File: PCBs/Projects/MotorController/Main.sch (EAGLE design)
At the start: 24 parts, among them Q1 ZXMP10A17GQ, Q2 BUK9240-100A.118, Q3 BUK9240-100A.118, Q4 MMBT5551LT1G, U1 LT4356-2

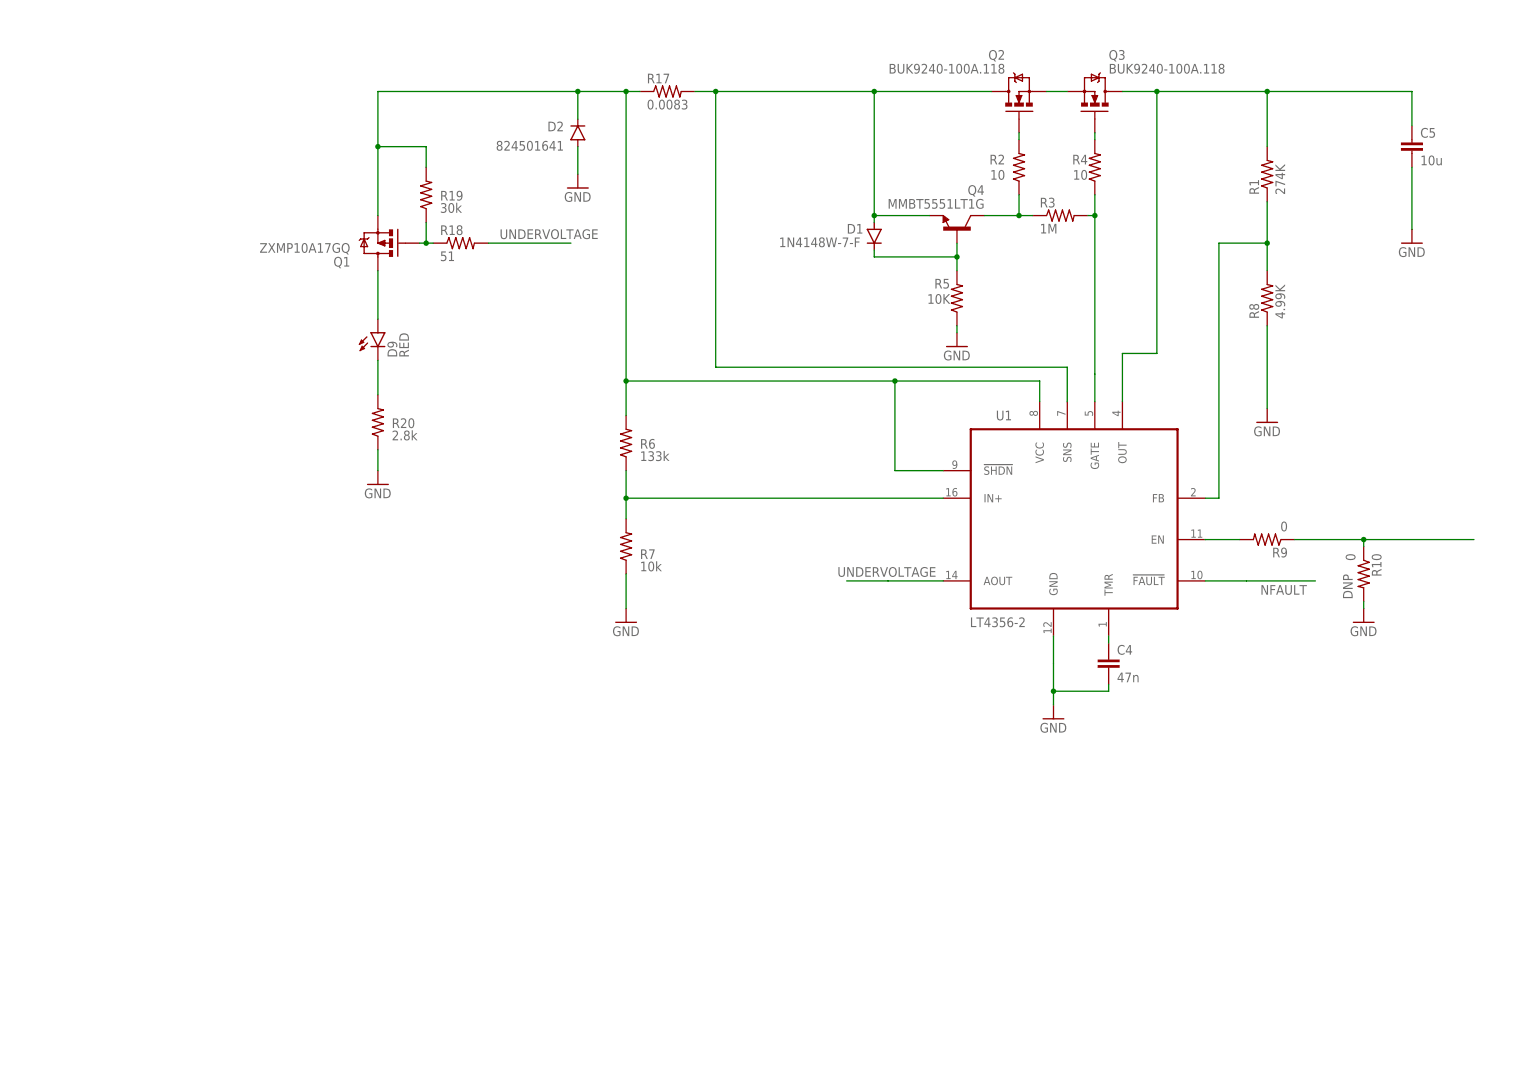
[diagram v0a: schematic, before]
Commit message: RepoFix
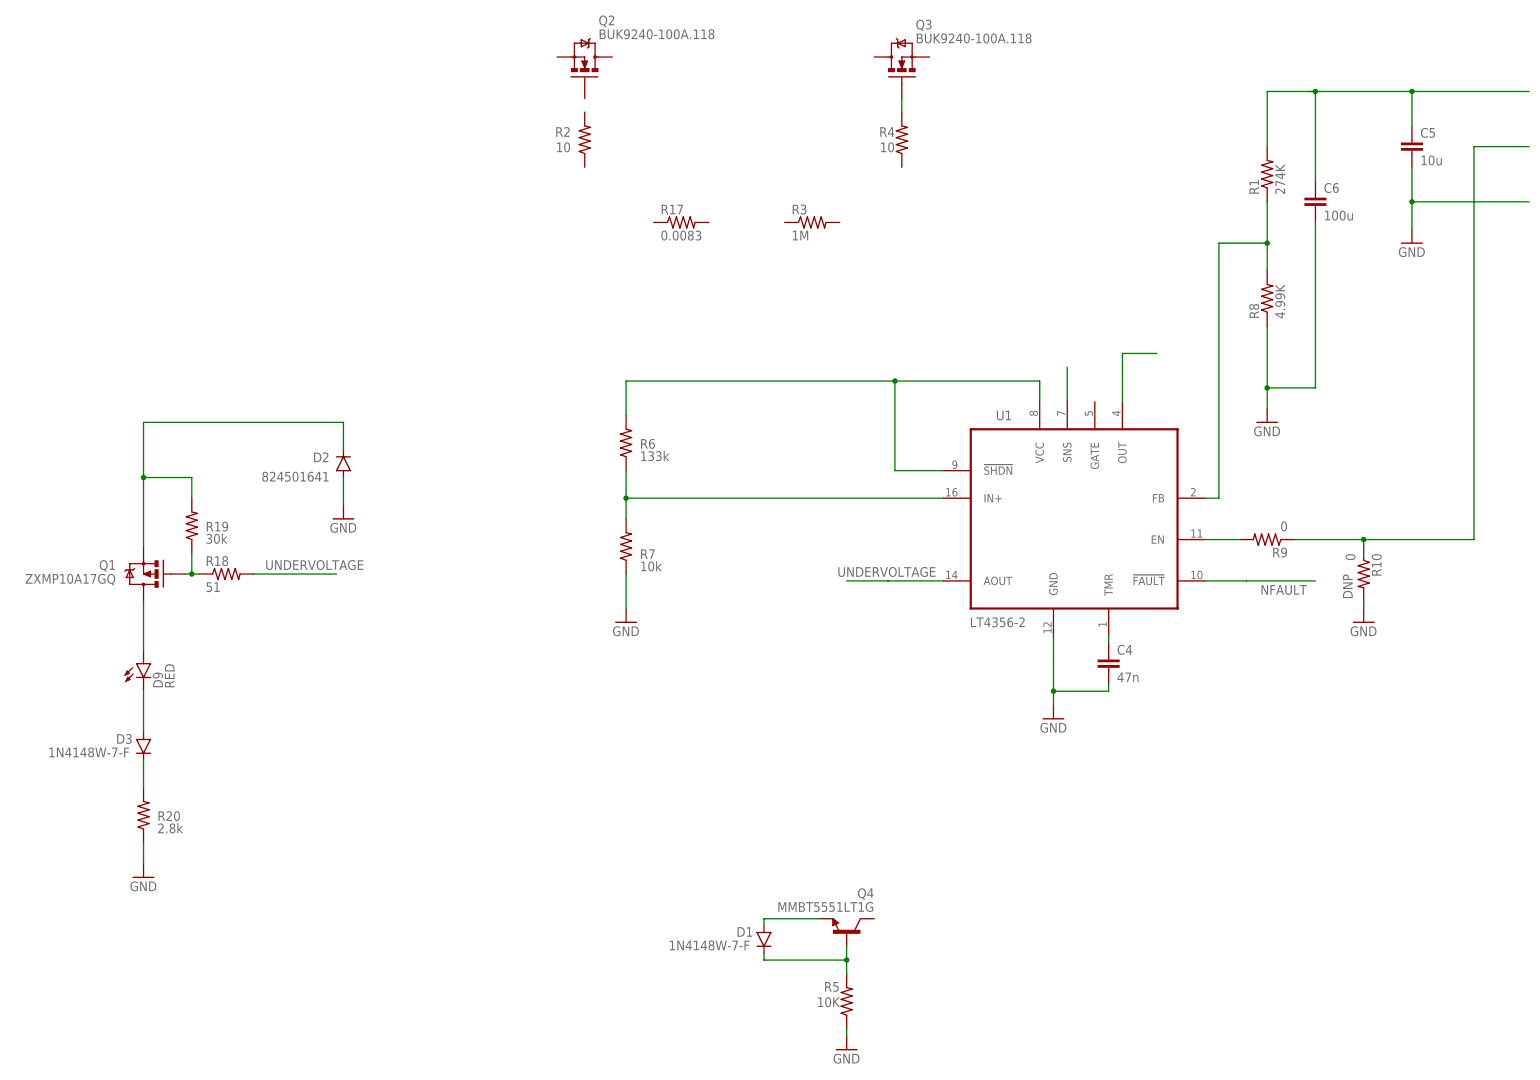
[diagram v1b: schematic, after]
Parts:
- added C6: 100u, SparkFun-Capacitors:CAP1210
- added D3: 1N4148W-7-F, SparkFun-DiscreteSemi:DIODESOD123
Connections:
- removed net N$10: Q2.G, R2.2
- removed net N$21: D9.C, R20.2
- removed net N$7: R3.2, R4.1, U1.GATE
- new net N$16: D3.C, R20.2
- new net N$17: U1.SNS
- new net N$4: D3.A, D9.C
- net GND: now also C6.2
- net N$12: no longer D2.C, Q1.S, R17.1, R19.2
- net N$3: now also C6.1; no longer Q3.D, U1.OUT
- net N$5: now also U1.OUT; no longer Q2.S, Q3.S
- net N$6: now also D2.C, Q1.S, R19.2; no longer Q4.C, R2.1, R3.1
- net N$8: no longer Q2.D, R17.2, U1.SNS
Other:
- moved on the sheet: D1, D2, D9, Q1, Q2, Q3, Q4, R17, R18, R19, R2, R20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
